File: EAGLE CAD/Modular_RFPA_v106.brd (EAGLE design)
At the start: 152.4 x 152.4 mm, 197 parts, among them IC301 74AHC1G14DBV, IC302 LM324D, J401 FUSE_2P, J402 KK_PCFAN, Q101 IRF520N, Q102 IRF630, Q201 IRF630, Q202 IRF630, Q301 BSS123, T101 HP4_TRAFO, T102 HP4_TRAFO, X402 HEATSINK_OMNI_DUAL30-75-D

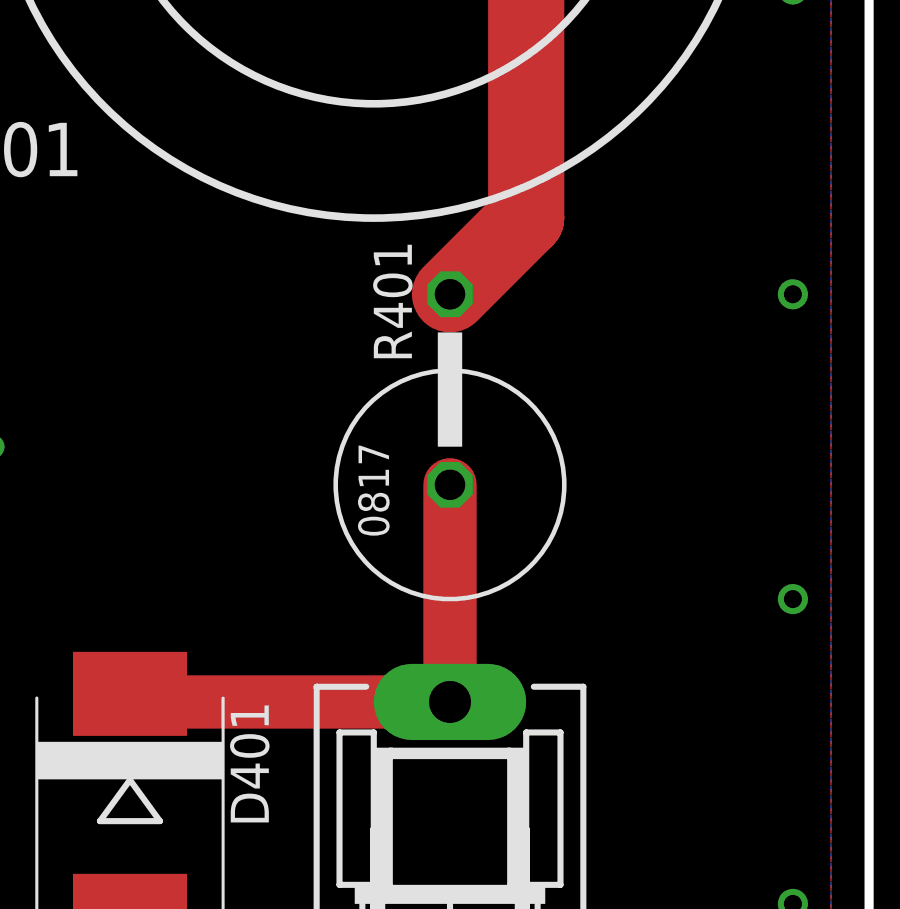
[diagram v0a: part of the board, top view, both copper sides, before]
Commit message: copy "R" variants to "R90"
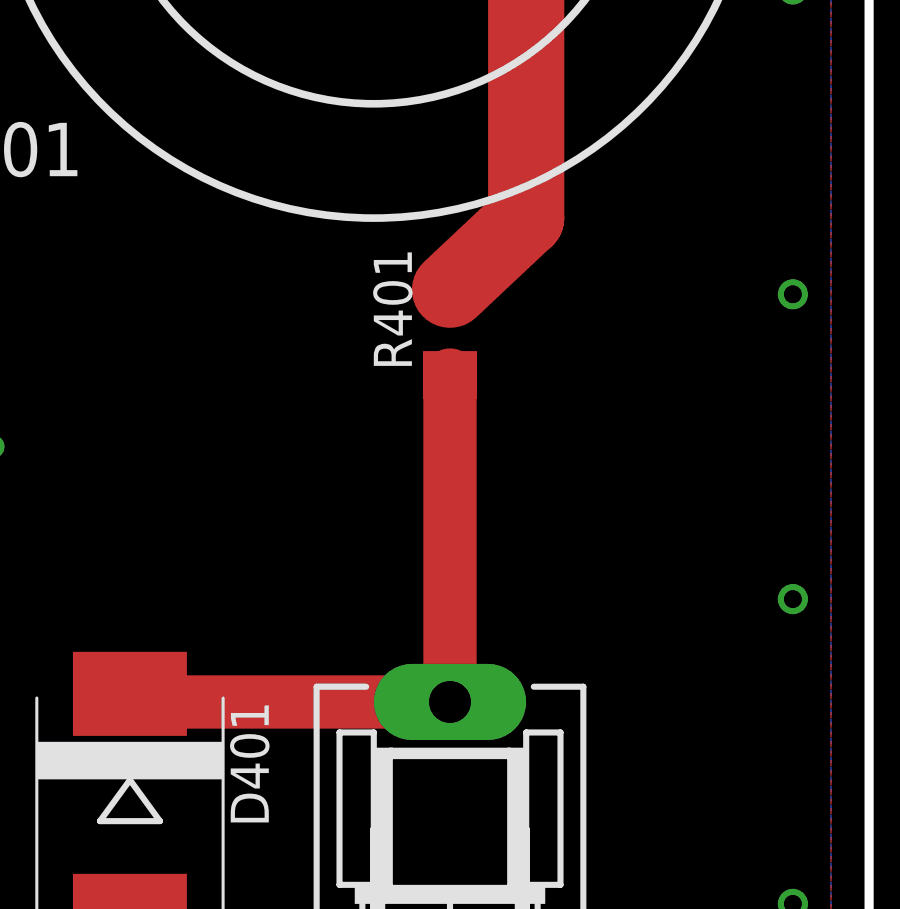
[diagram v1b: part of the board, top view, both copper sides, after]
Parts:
- R401: value (none) -> 1K; device resistor:P0817V -> MDT_R:R1206
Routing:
- net N$44: track 18.0 -> 21.7 mm
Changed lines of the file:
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@@
 <element name="IC402" library="v-reg" package="78XXS" value="" x="101.6" y="60.96" rot="R180"/>
 <element name="D401" library="diode" package="SMC" value="" x="127.762" y="31.242" rot="R270"/>
-<element name="R401" library="resistor" package="P0817V" value="" x="138.43" y="46.99" rot="R90"/>
+<element name="R401" library="MDT_R" package="R1206" value="1K" x="138.43" y="46.99" rot="R90">
+<attribute name="PACKAGE" value="1206" x="138.43" y="46.99" size="1.778" layer="27" rot="R90" display="off"/>
+<attribute name="PARTNO" value="" x="138.43" y="46.99" size="1.778" layer="27" rot="R90" display="off"/>
+<attribute name="BOM" value="" x="138.43" y="46.99" size="1.778" layer="27" rot="R90" display="off"/>
+<attribute name="TOL" value="1%" x="138.43" y="46.99" size="1.778" layer="27" rot="R90" display="off"/>
+<attribute name="VALUE" value="1K" x="138.43" y="46.99" size="1.778" layer="27" rot="R90" display="off"/>
+<attribute name="POWER" value="0.25" x="138.43" y="46.99" size="1.778" layer="27" rot="R90" display="off"/>
+</element>
 <element name="C401" library="rcl" package="EB25D" value="3300uF" x="135.89" y="63.5" rot="R180"/>
 <element name="C405" library="MDT_C" package="C2220_CKG57N" value="10uF" x="113.538" y="121.92" rot="R270">
@@
 <contactref element="R401" pad="1"/>
 <contactref element="J401" pad="2"/>
-<wire x1="138.43" y1="34.671" x2="138.43" y2="41.91" width="1.778" layer="1"/>
+<wire x1="138.43" y1="34.671" x2="138.43" y2="45.568" width="1.778" layer="1"/>
 <wire x1="138.43" y1="34.671" x2="128.033" y2="34.671" width="1.778" layer="1"/>
 <wire x1="128.033" y1="34.671" x2="127.762" y2="34.942" width="1.778" layer="1"/>
@@
 <contactref element="C401" pad="+"/>
 <contactref element="L401" pad="1"/>
-<wire x1="138.43" y1="48.26" x2="140.97" y2="50.8" width="2.54" layer="1"/>
+<wire x1="138.43" y1="48.412" x2="140.97" y2="50.8" width="2.54" layer="1"/>
 <wire x1="140.97" y1="50.8" x2="140.97" y2="63.5" width="2.54" layer="1"/>
 <wire x1="140.97" y1="63.5" x2="140.97" y2="91.948" width="2.54" layer="1"/>
